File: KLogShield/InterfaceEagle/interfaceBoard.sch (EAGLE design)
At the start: 10 parts, among them T1 2N2222, X1 1751280, X2 1751280, X3 1751303, X4 1751303, X5 1751303, X6 1751303, X7 1751248

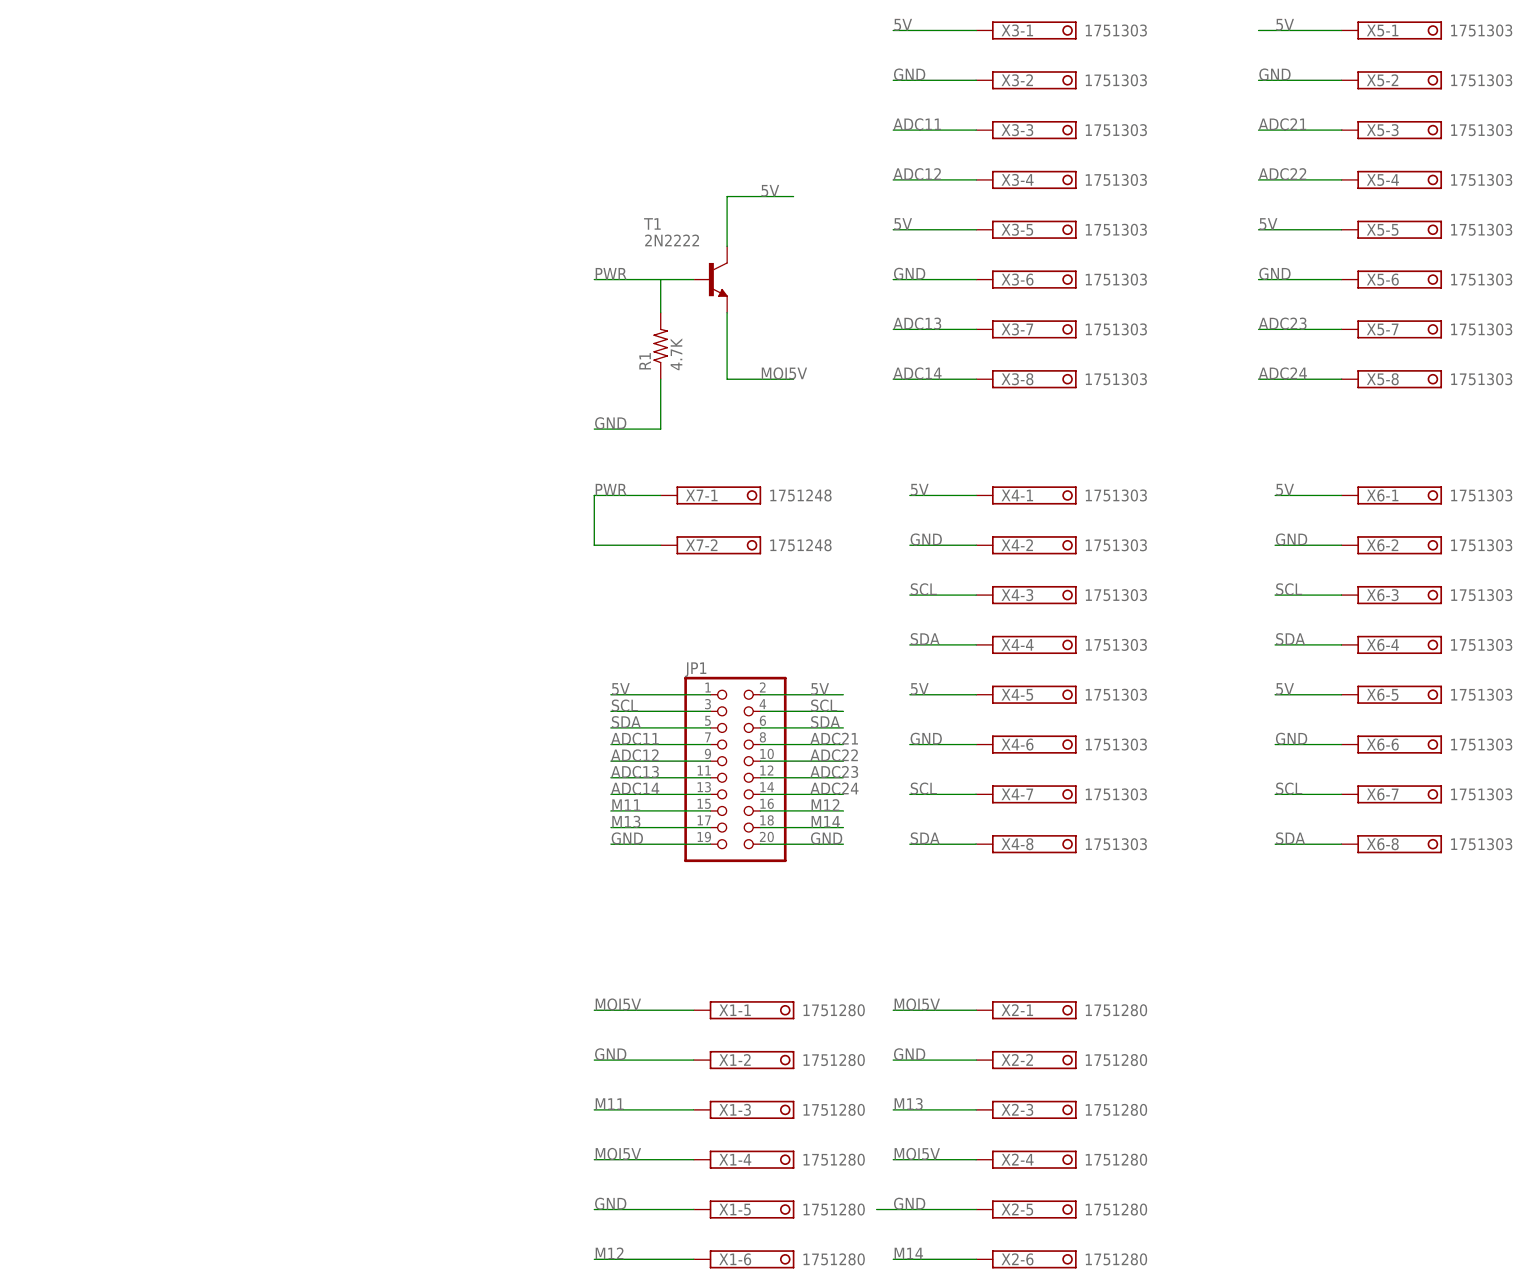
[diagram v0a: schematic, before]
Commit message: klog interface board gen2
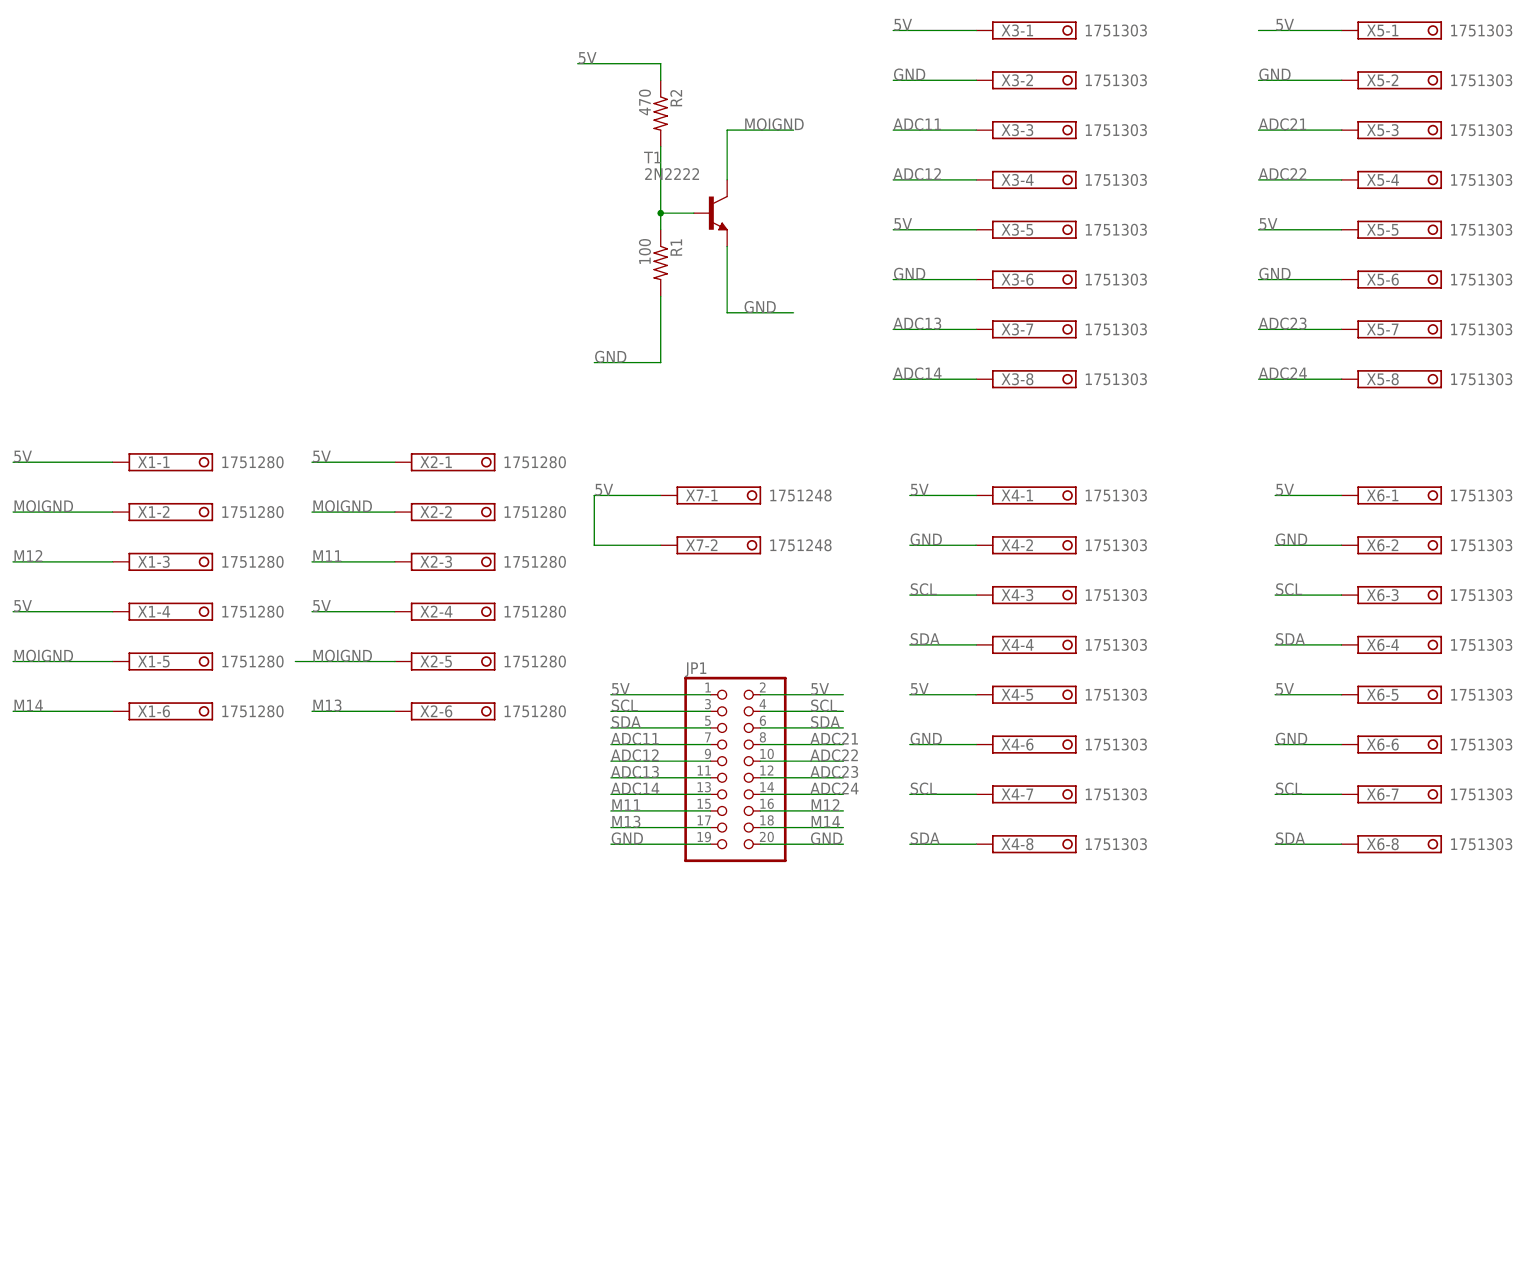
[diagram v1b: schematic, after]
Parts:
- added R2: 470, adafruit:R-US_M0805
- R1: value 4.7K -> 100; device adafruit:R-US_0207/9 -> adafruit:R-US_M0805
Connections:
- removed net MOI5V: T1.E, X1-1.K, X1-4.K, X2-1.K, X2-4.K
- removed net PWR: R1.2, T1.B, X7-1.K, X7-2.K
- new net MOIGND: T1.C, X1-2.K, X1-5.K, X2-2.K, X2-5.K
- new net N$7: R1.1, R2.2, T1.B
- net 5V: now also R2.1, X1-1.K, X1-4.K, X2-1.K, X2-4.K, X7-1.K, X7-2.K; no longer T1.C
- net GND: now also R1.2, T1.E; no longer R1.1, X1-2.K, X1-5.K, X2-2.K, X2-5.K
- net M11: now also X2-3.K; no longer X1-3.K
- net M12: now also X1-3.K; no longer X1-6.K
- net M13: now also X2-6.K; no longer X2-3.K
- net M14: now also X1-6.K; no longer X2-6.K
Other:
- moved on the sheet: R1, T1, X1-1, X1-2, X1-3, X1-4, X1-5, X1-6, X2-1, X2-2, X2-3, X2-4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
